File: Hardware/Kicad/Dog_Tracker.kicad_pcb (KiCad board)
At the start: 2 copper layers, 21 parts, among them IC1 M4 Feather, U1 ADP160AUJZ-1.8-R7, U2 SX1280IMLTRT, U3 Origin_GPS1510, U4 NFA18SL407V1A45L, U5 SN74AUP1T97, U6 LSM6DSO32

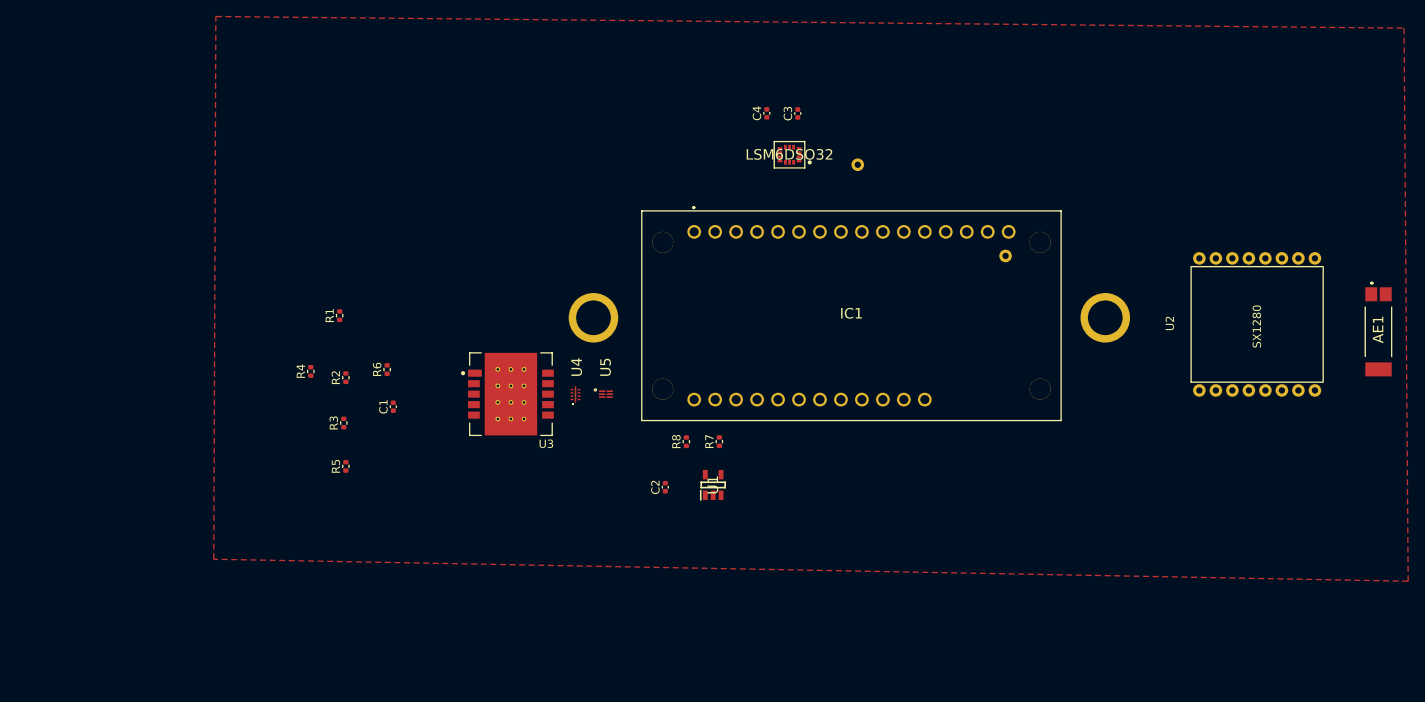
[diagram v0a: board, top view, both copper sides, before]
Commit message: pcb check
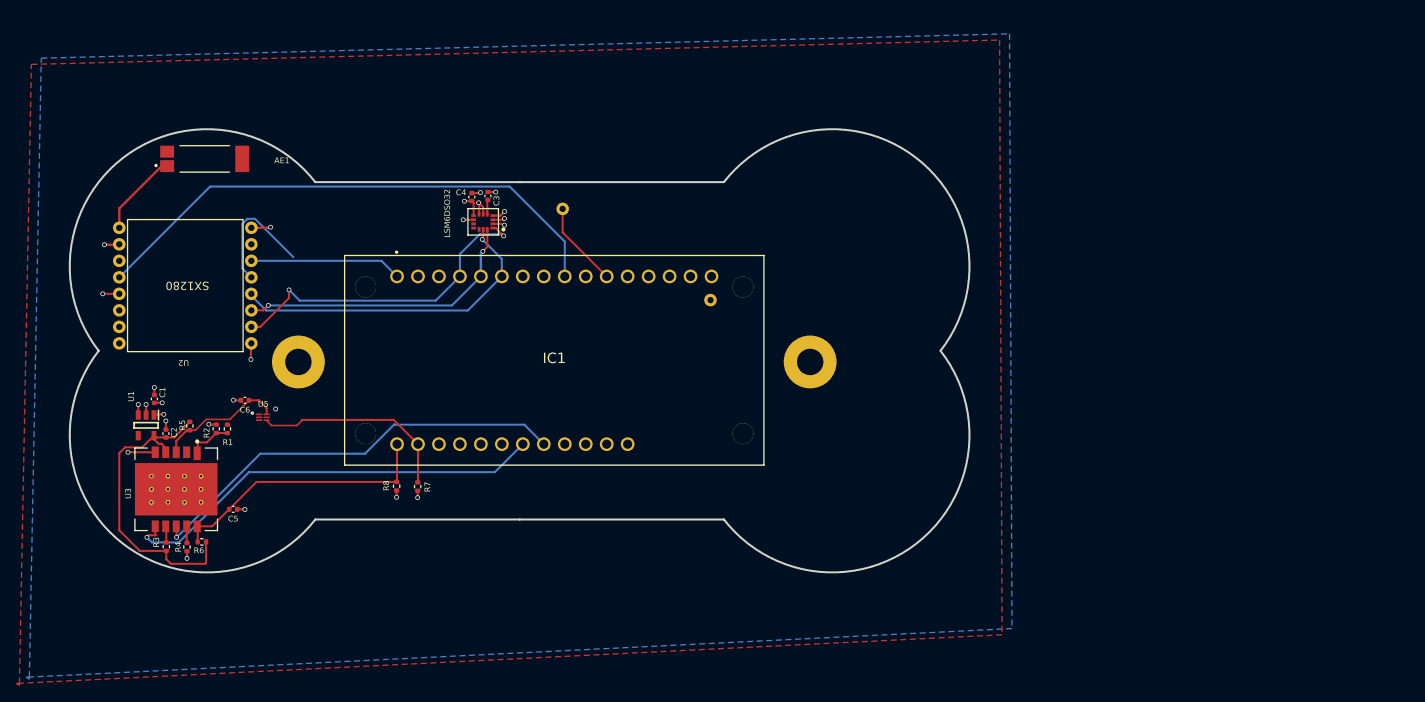
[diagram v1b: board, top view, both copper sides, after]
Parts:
- removed U4: NFA18SL407V1A45L, Dog_Tracker:NFA18SL307V1A45B
- added C5: 22pF, Capacitor_SMD:C_0402_1005Metric, F.Cu at (61.4, 122.0)
- added C6: 22pF, Capacitor_SMD:C_0402_1005Metric, F.Cu at (62.8, 108.8)
- moved AE1 143.7 mm to (57.9, 79.5), turned to 180 degrees
- moved U2 129.9 mm to (55.5, 94.8), turned to 180 degrees
- moved U1 69.1 mm to (50.8, 111.8), turned to -90 degrees
- moved C2 60.8 mm to (53.2, 112.8)
- moved U3 42.2 mm to (54.4, 119.5), turned to 90 degrees
- moved U5 41.7 mm to (64.9, 110.8)
- moved C3 38.8 mm to (92.2, 84.0)
- moved U6 38.0 mm to (91.6, 87.1)
- moved C4 37.1 mm to (90.3, 84.1)
- moved R7 37.0 mm to (83.7, 119.2), turned to -90 degrees
- moved IC1 36.4 mm to (100.2, 103.7)
- moved LS1 36.1 mm to (100.2, 104.1)
- moved R8 35.5 mm to (81.2, 119.2), turned to -90 degrees
- moved R6 30.7 mm to (57.6, 125.9), turned to 0 degrees
- moved C1 29.0 mm to (51.8, 108.6)
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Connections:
- net Net-(AE1-Pad1) renamed /ANT
- net Net-(IC1-Pad4) renamed /MISO
- net Net-(IC1-Pad5) renamed /MOSI
- net Net-(IC1-Pad6) renamed /SCK
- net Net-(IC1-Pad9) renamed /BUSY
- net Net-(R3-Pad1) renamed /CTS
- net Net-(R4-Pad1) renamed /RTS
- R5 pad 1: Net-(R5-Pad1) -> Net-(C6-Pad1)
- R6 pad 1: Net-(R6-Pad1) -> /I2C_SDA
- U3 pad 10: Net-(R6-Pad1) -> /I2C_SDA
- U3 pad 3: Net-(R5-Pad1) -> Net-(C6-Pad1)
- U5 pad 1: Net-(U4-Pad9) -> Net-(C6-Pad1)
- U5 pad 3: Net-(U4-Pad9) -> Net-(C6-Pad1)
- U5 pad 6: Net-(U4-Pad9) -> Net-(C6-Pad1)
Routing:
- net +3V3: track 0.00 -> 177.6 mm, vias 0 -> 8
- net /BUSY: track 0.00 -> 65.5 mm
- net /wakeup: track 0.00 -> 53.0 mm, vias 0 -> 1
- net /gps reset: track 0.00 -> 52.5 mm, vias 0 -> 1
- net /MISO: track 0.00 -> 40.2 mm, vias 0 -> 2
- net /SCK: track 0.00 -> 39.8 mm, vias 0 -> 1
- net +1V8: track 0.00 -> 38.1 mm
- net /MOSI: track 0.00 -> 35.5 mm, vias 0 -> 2
- net /I2C_SDA: track 0.00 -> 32.8 mm
- net GND: track 0.00 -> 27.1 mm, vias 0 -> 18
- net /I2C_SCL: track 0.00 -> 24.7 mm
- net /lora reset: track 0.00 -> 18.4 mm
- net Net-(C6-Pad1): track 0.00 -> 15.7 mm
- net /lora cs: track 0.00 -> 15.3 mm
- net Net-(IC1-Pad11): track 0.00 -> 10.4 mm
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- added copper zone on B.Cu, net (none)
- added copper zone on F.Cu, net (none)
- added copper zone on In2.Cu, net +3V3
- added copper zone on In1.Cu, net GND
- removed copper zone on F.Cu, net GND
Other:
- board outline added: 109 x 53.7 mm
- copper layers 2 -> 4
